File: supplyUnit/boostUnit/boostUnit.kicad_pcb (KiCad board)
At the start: 2 copper layers, 72.7 x 33.9 mm, 26 parts, among them J1 Conn_02x03_Counter_Clockwise, J2 Conn_02x03_Counter_Clockwise

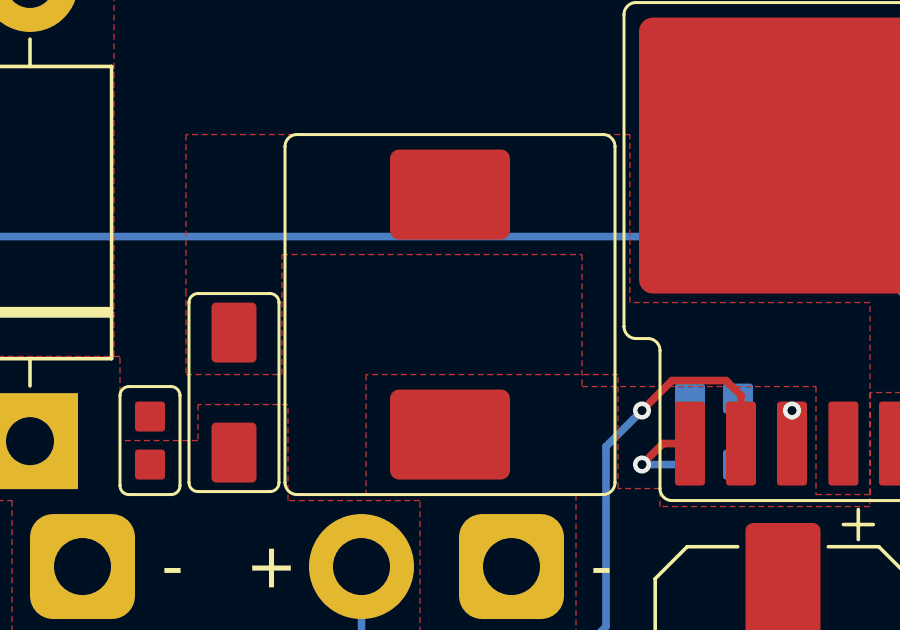
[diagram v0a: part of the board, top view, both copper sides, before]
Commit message: 死
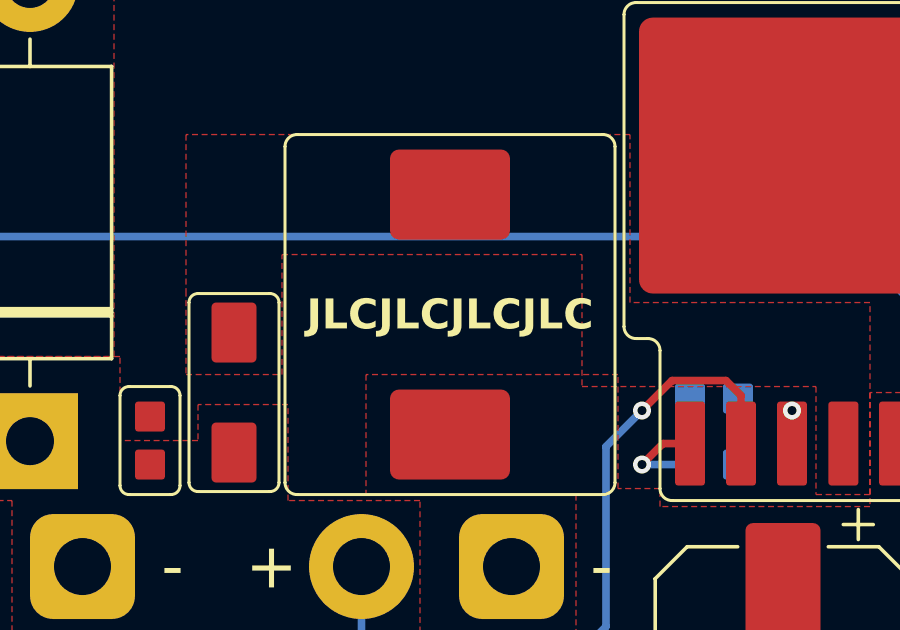
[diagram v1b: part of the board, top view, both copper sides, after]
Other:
- board text added: "JLCJLCJLCJLC"
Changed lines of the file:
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@@
+		)
+	)
+	(gr_text "JLCJLCJLCJLC"
+		(at 144.780978 100.183123 0)
+		(layer "F.SilkS")
+		(effects
+			(font
+				(size 1 1)
+				(thickness 0.25)
+				(bold yes)
+			)
 		)
 	)
